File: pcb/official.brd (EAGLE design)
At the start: 114.3 x 55.5 mm, 22 parts, among them IC1 LM386N-4, P1 DEV_CLP-150, P8 DEV_1X40

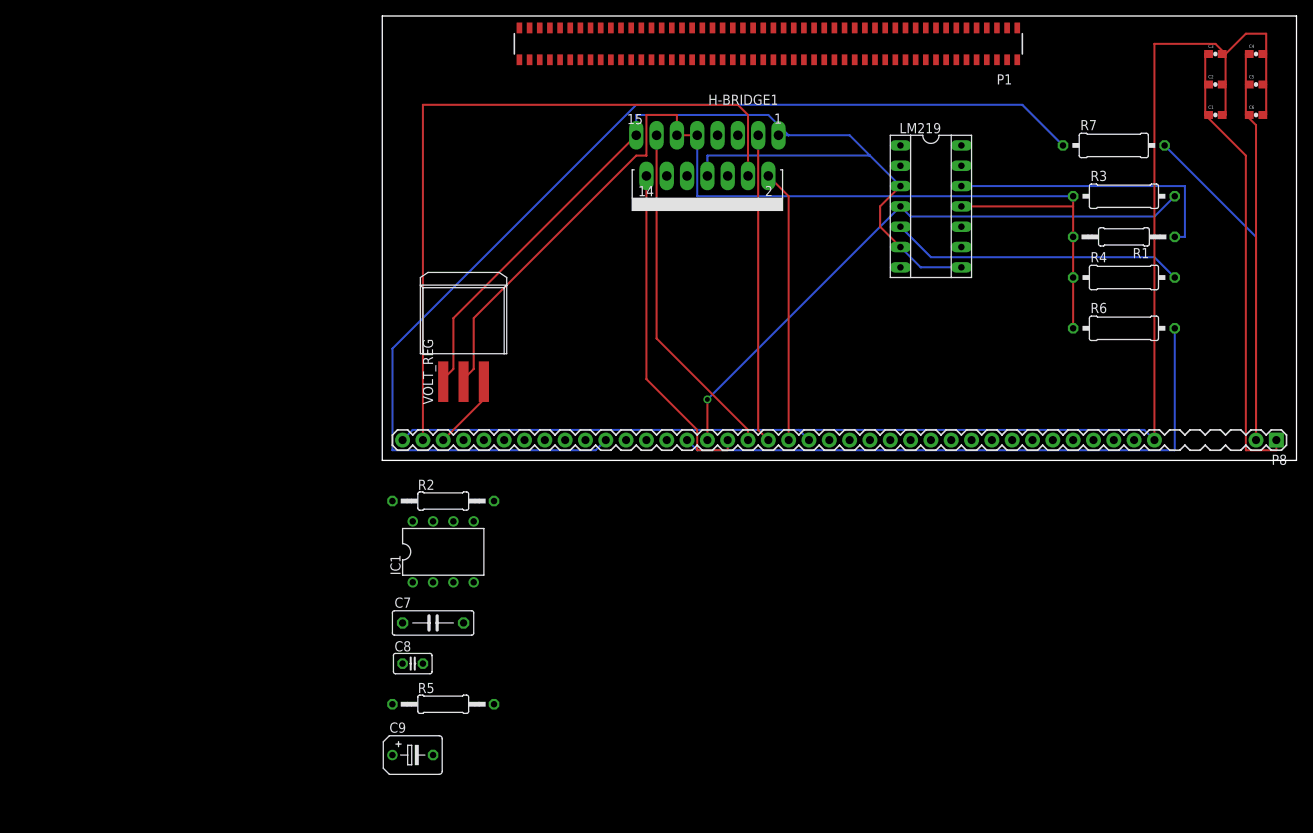
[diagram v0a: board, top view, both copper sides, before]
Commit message: Better pcb
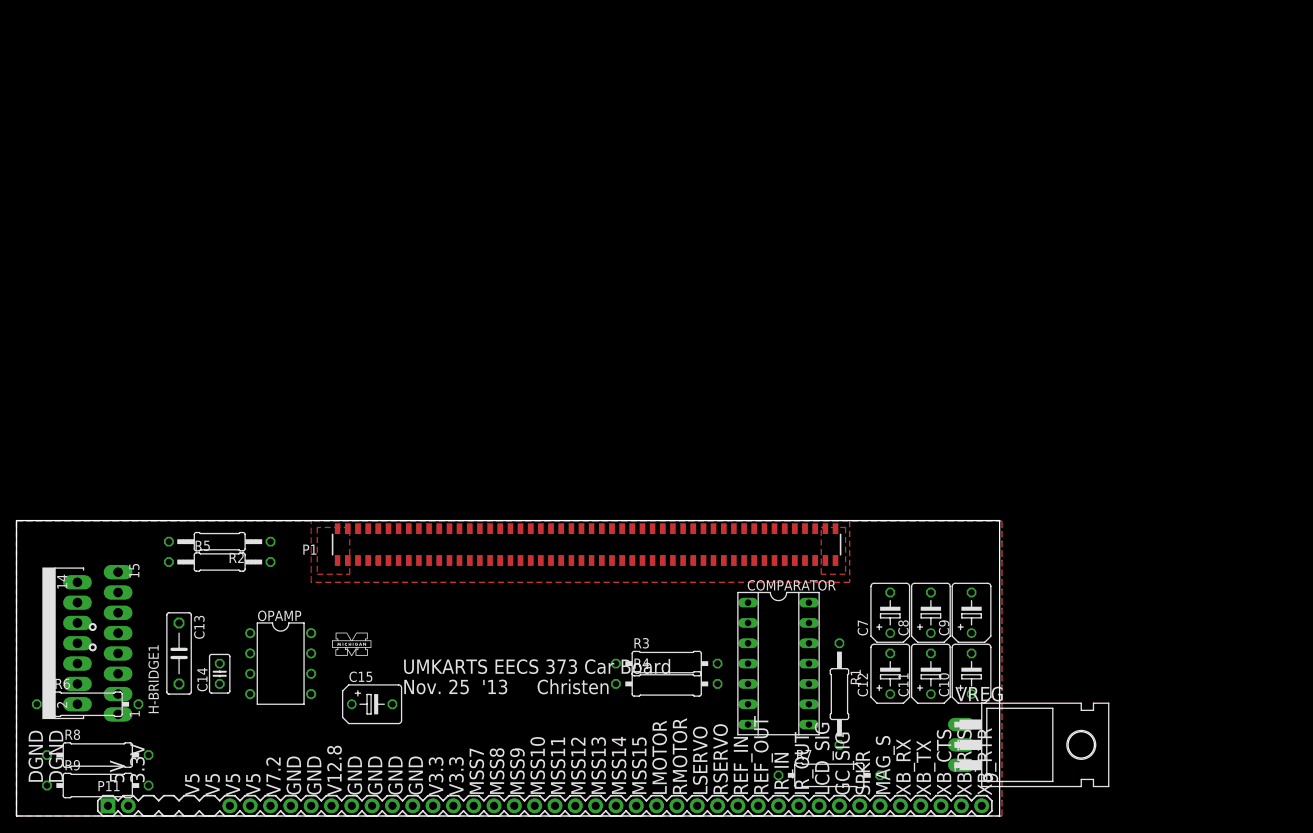
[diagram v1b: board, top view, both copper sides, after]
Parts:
- removed C1, C2, C3, C4, C5, C6: (no value), SparkFun:0603-CAP
- removed IC1: LM386N-4, linear:DIL08
- removed LM219: (no value), ic-package:SOCKET-14
- removed P8: DEV_1X40, EECS370:1X40
- removed VOLT_REG: REG1117F, burr-brown:DD-3
- added C10, C11, C12, C15: (no value), rcl:B45181B
- added C13: (no value), rcl:C075-032X103
- added C14: (no value), rcl:C025-025X050
- added COMPARATOR: (no value), ic-package:SOCKET-14
- added OPAMP: LM386N-4, linear:DIL08
- added P11: DEV_1X40, EECS370:1X40
- added R8: 750, rcl:0309/12
- added R9: 10, rcl:0309/12
- added U$1: (no value), umich:UMICH
- added VREG: 7806T, linear:TO220H
- C7: device rcl:C075-032X103 -> rcl:B45181B
- C8: device rcl:C025-025X050 -> rcl:B45181B
- moved R6 137.8 mm to (8.89, 14.0)
- moved H-BRIDGE1 98.6 mm to (5.08, 21.6), turned to 90 degrees
- moved R7 86.4 mm to (101.6, 5.08)
- moved R3 81.7 mm to (81.3, 19.1)
- moved R4 76.5 mm to (81.3, 16.5)
- moved C9 72.1 mm to (119.4, 25.4), turned to 90 degrees
- moved R1 67.3 mm to (102.9, 15.2), turned to 270 degrees
- moved P1 66.6 mm to (71.3, 33.9), turned to 0 degrees
- moved C8 65.1 mm to (114.3, 25.4), turned to 90 degrees
- moved C7 57.2 mm to (109.2, 25.4), turned to 90 degrees
- moved R5 33.1 mm to (25.4, 31.8)
- moved R2 28.4 mm to (25.4, 34.3), turned to 180 degrees
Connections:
- removed net 5V: H-BRIDGE1.11, H-BRIDGE1.9, LM219.11, R1.2, R3.1, R4.1, R6.1, VOLT_REG.2
- removed net GND: H-BRIDGE1.1, H-BRIDGE1.15, H-BRIDGE1.8, IC1.2, IC1.4, LM219.3, LM219.6, LM219.8, R2.1, R5.2, VOLT_REG.1
- new net ADC11: P1.P$90
- new net ADC9: P1.P$86
- new net MSS_GPIO_5: P11.39
- new net MSS_GPIO_6: P11.40
- new net N$1: H-BRIDGE1.13, R9.2
- net 12.8V: no longer P8.39
- net 7.2V: now also VREG.1; no longer P8.38, VOLT_REG.3
- net ADC0: no longer P8.35
- net ADC1: no longer P8.36
- net ADC4: no longer P8.33
- net ADC5: no longer P8.34
- net ADC6: no longer P8.37
- net ADC8: no longer P8.32
- net AGND: now also P1.P$88, P1.P$92, P1.P$94
- net DACOUT1: now also C13.2; no longer C7.2
- net DGND: now also C10.-, C11.-, C12.-, C7.-, C8.-, C9.-, COMPARATOR.3, COMPARATOR.6, COMPARATOR.8, H-BRIDGE1.1, H-BRIDGE1.15, H-BRIDGE1.8, OPAMP.2, OPAMP.4, P1.P$96, P11.9, R2.1, R5.2, VREG.2; no longer C1.2, C2.2, C3.2, C4.2, C5.2, C6.2, P8.20, P8.3, P8.40
- net F2-200-IO_0: now also P11.30; no longer H-BRIDGE1.6
- net F2-200-IO_1: now also P11.31; no longer P8.29
- net F2-200-IO_2: now also P11.32; no longer P8.30, R7.1
- net F2-200-IO_3: now also P11.33, R7.1; no longer H-BRIDGE1.5
- net F2-200-IO_4: now also H-BRIDGE1.6; no longer H-BRIDGE1.7
- net F2-200-IO_5: now also H-BRIDGE1.5; no longer P8.28
- net F2-200-IO_6: now also H-BRIDGE1.7; no longer H-BRIDGE1.10
- net F2-200-IO_7: now also H-BRIDGE1.10; no longer H-BRIDGE1.12
- net F2-200-IO_8: now also H-BRIDGE1.12; no longer P8.27
- net LMOTOR: now also P11.24; no longer P8.21
- net LSERVO: now also P11.26, R9.1; no longer H-BRIDGE1.13, P8.23
- net MSS_GP_IO_0: now also P11.35, R8.2; no longer P8.4
- net MSS_GP_IO_1: now also COMPARATOR.12, R1.1; no longer P8.5
- net MSS_GP_IO_10: now also P11.18; no longer P8.14
- net MSS_GP_IO_11: now also P11.19; no longer P8.15
- net MSS_GP_IO_12: now also P11.20; no longer P8.16
- net MSS_GP_IO_13: now also P11.21; no longer P8.17
- net MSS_GP_IO_14: now also P11.22; no longer P8.18
- net MSS_GP_IO_15: now also P11.23; no longer P8.19
- net MSS_GP_IO_2: now also P11.36; no longer LM219.12, R1.1
- net MSS_GP_IO_3: now also P11.37; no longer P8.7
- net MSS_GP_IO_4: now also P11.38; no longer P8.8
- net MSS_GP_IO_5: no longer P8.9
- net MSS_GP_IO_6: no longer P8.10
- net MSS_GP_IO_7: now also P11.15; no longer P8.11
- net MSS_GP_IO_8: now also P11.16; no longer P8.12
- net MSS_GP_IO_9: now also P11.17; no longer P8.13
- net N$2: now also C13.1, OPAMP.3; no longer C7.1, IC1.3
- net N$3: now also COMPARATOR.5; no longer LM219.5
- net N$4: now also C14.2; no longer C8.2
- net N$5: now also C14.1, C15.+, OPAMP.5; no longer C8.1, C9.+, IC1.5
- net N$6: now also OPAMP.6; no longer IC1.6
- net REFS_IN: now also COMPARATOR.4, P11.28, R3.2; no longer P8.26, R6.2
- net REFS_OUT: now also P11.29, R6.2; no longer LM219.4, P8.25, R3.2
- net RMOTOR: now also P11.25; no longer P8.22
- net RSERVO: now also P11.27; no longer P8.24
- net SPKR: now also C15.-, P11.34; no longer C9.-, P8.31
- net VDD3.3: now also C10.+, C11.+, C12.+, P1.P$100, P1.P$98, P11.14; no longer C4.1, C5.1, C6.1, P8.2
- net VDD5: now also C7.+, C8.+, C9.+, COMPARATOR.11, H-BRIDGE1.11, H-BRIDGE1.9, P11.1, P11.4, R1.2, R3.1, R4.1, R6.1, R8.1, VREG.3; no longer C1.1, C2.1, C3.1, P8.1
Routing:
- net DGND: track 182.2 -> 0.00 mm
- net F2-200-IO_2: track 138.4 -> 0.00 mm
- net 5V: track 137.5 -> 0.00 mm
- net GND: track 122.6 -> 0.00 mm
- net VDD3.3: track 91.6 -> 0.00 mm
- net 12.8V: track 90.7 -> 0.00 mm
- net REFS_IN: track 76.7 -> 0.00 mm
- net REFS_OUT: track 75.1 -> 0.00 mm, vias 1 -> 0
- net VDD5: track 58.0 -> 0.00 mm
- net LSERVO: track 42.8 -> 0.00 mm
- net RSERVO: track 42.0 -> 0.00 mm
- net RMOTOR: track 38.6 -> 0.00 mm
- net N$3: track 36.9 -> 0.00 mm
- net MSS_GP_IO_2: track 35.6 -> 0.00 mm
- net LMOTOR: track 34.1 -> 0.00 mm
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- added copper zone on layer 16, net N$7
- added copper zone on layer 1, net N$8
- added copper zone on layer 1, net VDD3.3
- added copper zone on layer 1, net VDD5
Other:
- board size 114.3 x 55.5 mm -> 122.9 x 36.9 mm
- board text added: "3.3V"
- board text added: "5V"
- board text added: "9"
- board text added: "DGND"
- board text added: "GC_SIG"
- board text added: "GND"
- board text added: "IR_IN"
- board text added: "IR_OUT"
- board text added: "LCD_SIG"
- board text added: "LMOTOR"
- board text added: "LSERVO"
- board text added: "MAG_S"
- board text added: "MSS10"
- board text added: "MSS11"
- board text added: "MSS12"
- board text added: "MSS13"
- board text added: "MSS14"
- board text added: "MSS15"
- board text added: "MSS7"
- board text added: "MSS8"
- board text added: "MSS9"
- board text added: "Nov. 25 '13 Christen"
- board text added: "REF_IN"
- board text added: "REF_OUT"
- board text added: "RMOTOR"
- board text added: "RSERVO"
- board text added: "SPKR"
- board text added: "UMKARTS EECS 373 Car Board"
- board text added: "V12.8"
- board text added: "V3.3"
- board text added: "V5"
- board text added: "V7.2"
- board text added: "XB_CTS"
- board text added: "XB_RTR"
- board text added: "XB_RTS"
- board text added: "XB_RX"
- board text added: "XB_TX"
